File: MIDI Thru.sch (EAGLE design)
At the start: 49 parts, among them IC1 6N136, IC2 6N136, IC3 6N136, IC5 74HCT14, T1 2N3904, U1 7805T

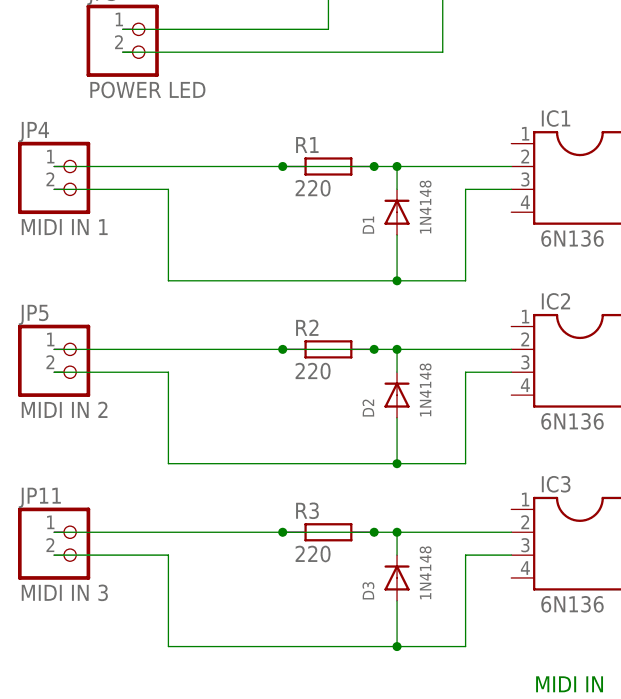
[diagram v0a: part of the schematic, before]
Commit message: updating schematic
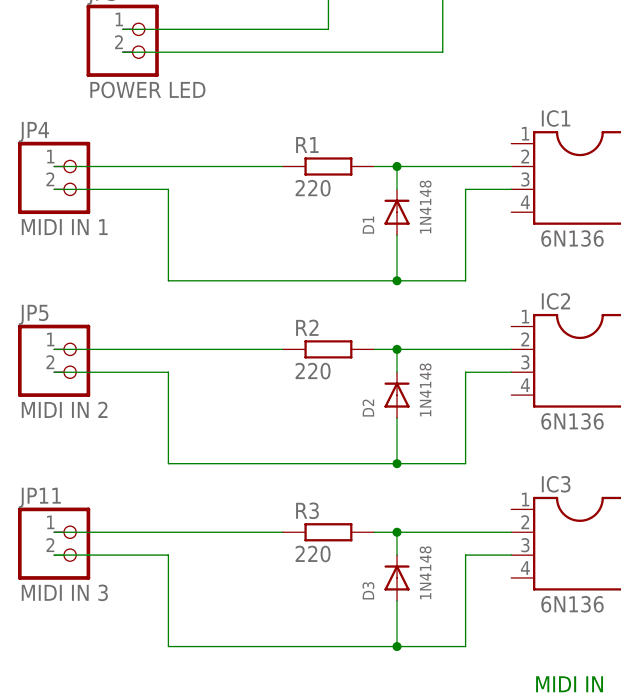
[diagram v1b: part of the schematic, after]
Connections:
- new net N$12: D3.C, IC3.2, R3.2
- new net N$7: JP4.1, R1.1
- new net N$9: D2.C, IC2.2, R2.2
- net N$1: no longer JP4.1, R1.1
- net N$3: no longer D2.C, IC2.2, R2.2
- net N$5: no longer D3.C, IC3.2, R3.2
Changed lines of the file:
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@@
 <net name="N$1" class="0">
 <segment>
-<pinref part="JP4" gate="G$1" pin="1"/>
-<wire x1="-73.66" y1="114.3" x2="-48.26" y2="114.3" width="0.1524" layer="91"/>
 <pinref part="IC1" gate="G$1" pin="2"/>
 <pinref part="D1" gate="G$1" pin="C"/>
-<wire x1="-48.26" y1="114.3" x2="-38.1" y2="114.3" width="0.1524" layer="91"/>
 <wire x1="-38.1" y1="114.3" x2="-35.56" y2="114.3" width="0.1524" layer="91"/>
 <wire x1="-35.56" y1="114.3" x2="-22.86" y2="114.3" width="0.1524" layer="91"/>
 <wire x1="-35.56" y1="111.76" x2="-35.56" y2="114.3" width="0.1524" layer="91"/>
 <junction x="-35.56" y="114.3"/>
-<pinref part="R1" gate="G$1" pin="1"/>
-<junction x="-48.26" y="114.3"/>
 <pinref part="R1" gate="G$1" pin="2"/>
-<junction x="-38.1" y="114.3"/>
 </segment>
 </net>
@@
 <pinref part="JP5" gate="G$1" pin="1"/>
 <wire x1="-73.66" y1="93.98" x2="-48.26" y2="93.98" width="0.1524" layer="91"/>
-<pinref part="IC2" gate="G$1" pin="2"/>
-<pinref part="D2" gate="G$1" pin="C"/>
-<wire x1="-48.26" y1="93.98" x2="-38.1" y2="93.98" width="0.1524" layer="91"/>
-<wire x1="-38.1" y1="93.98" x2="-35.56" y2="93.98" width="0.1524" layer="91"/>
-<wire x1="-35.56" y1="93.98" x2="-22.86" y2="93.98" width="0.1524" layer="91"/>
-<wire x1="-35.56" y1="91.44" x2="-35.56" y2="93.98" width="0.1524" layer="91"/>
-<junction x="-35.56" y="93.98"/>
 <pinref part="R2" gate="G$1" pin="1"/>
-<junction x="-48.26" y="93.98"/>
-<pinref part="R2" gate="G$1" pin="2"/>
-<junction x="-38.1" y="93.98"/>
 </segment>
 </net>
@@
 <pinref part="JP11" gate="G$1" pin="1"/>
 <wire x1="-73.66" y1="73.66" x2="-48.26" y2="73.66" width="0.1524" layer="91"/>
-<pinref part="IC3" gate="G$1" pin="2"/>
-<pinref part="D3" gate="G$1" pin="C"/>
-<wire x1="-48.26" y1="73.66" x2="-38.1" y2="73.66" width="0.1524" layer="91"/>
-<wire x1="-38.1" y1="73.66" x2="-35.56" y2="73.66" width="0.1524" layer="91"/>
-<wire x1="-35.56" y1="73.66" x2="-22.86" y2="73.66" width="0.1524" layer="91"/>
-<wire x1="-35.56" y1="71.12" x2="-35.56" y2="73.66" width="0.1524" layer="91"/>
-<junction x="-35.56" y="73.66"/>
 <pinref part="R3" gate="G$1" pin="1"/>
-<junction x="-48.26" y="73.66"/>
-<pinref part="R3" gate="G$1" pin="2"/>
-<junction x="-38.1" y="73.66"/>
 </segment>
 </net>
@@
 </segment>
 </net>
+<net name="N$7" class="0">
+<segment>
+<pinref part="R1" gate="G$1" pin="1"/>
+<pinref part="JP4" gate="G$1" pin="1"/>
+<wire x1="-48.26" y1="114.3" x2="-73.66" y2="114.3" width="0.1524" layer="91"/>
+</segment>
+</net>
+<net name="N$9" class="0">
+<segment>
+<pinref part="IC2" gate="G$1" pin="2"/>
+<wire x1="-35.56" y1="93.98" x2="-22.86" y2="93.98" width="0.1524" layer="91"/>
+<pinref part="D2" gate="G$1" pin="C"/>
+<wire x1="-35.56" y1="91.44" x2="-35.56" y2="93.98" width="0.1524" layer="91"/>
+<junction x="-35.56" y="93.98"/>
+<wire x1="-38.1" y1="93.98" x2="-35.56" y2="93.98" width="0.1524" layer="91"/>
+<pinref part="R2" gate="G$1" pin="2"/>
+</segment>
+</net>
+<net name="N$12" class="0">
+<segment>
+<pinref part="IC3" gate="G$1" pin="2"/>
+<wire x1="-35.56" y1="73.66" x2="-22.86" y2="73.66" width="0.1524" layer="91"/>
+<pinref part="D3" gate="G$1" pin="C"/>
+<wire x1="-35.56" y1="71.12" x2="-35.56" y2="73.66" width="0.1524" layer="91"/>
+<junction x="-35.56" y="73.66"/>
+<wire x1="-38.1" y1="73.66" x2="-35.56" y2="73.66" width="0.1524" layer="91"/>
+<pinref part="R3" gate="G$1" pin="2"/>
+</segment>
+</net>
